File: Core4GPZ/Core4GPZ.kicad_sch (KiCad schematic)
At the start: 3 parts, among them U1 core4, U2 MPX4250

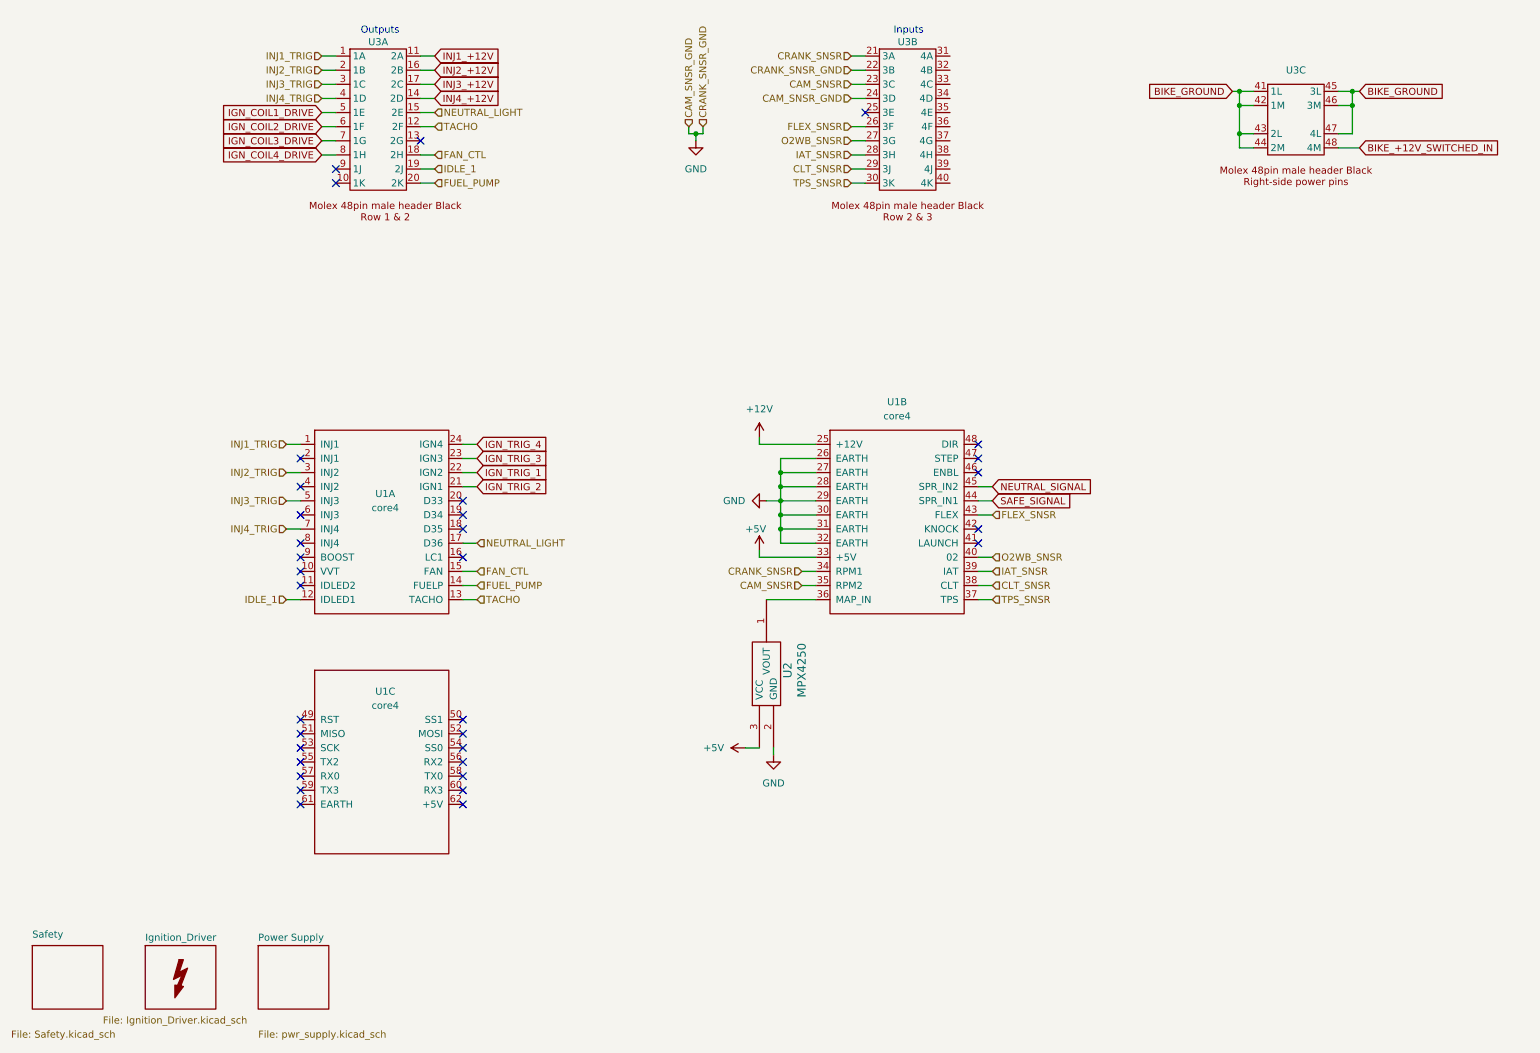
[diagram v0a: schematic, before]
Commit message: Test montage générateur de Haute tension
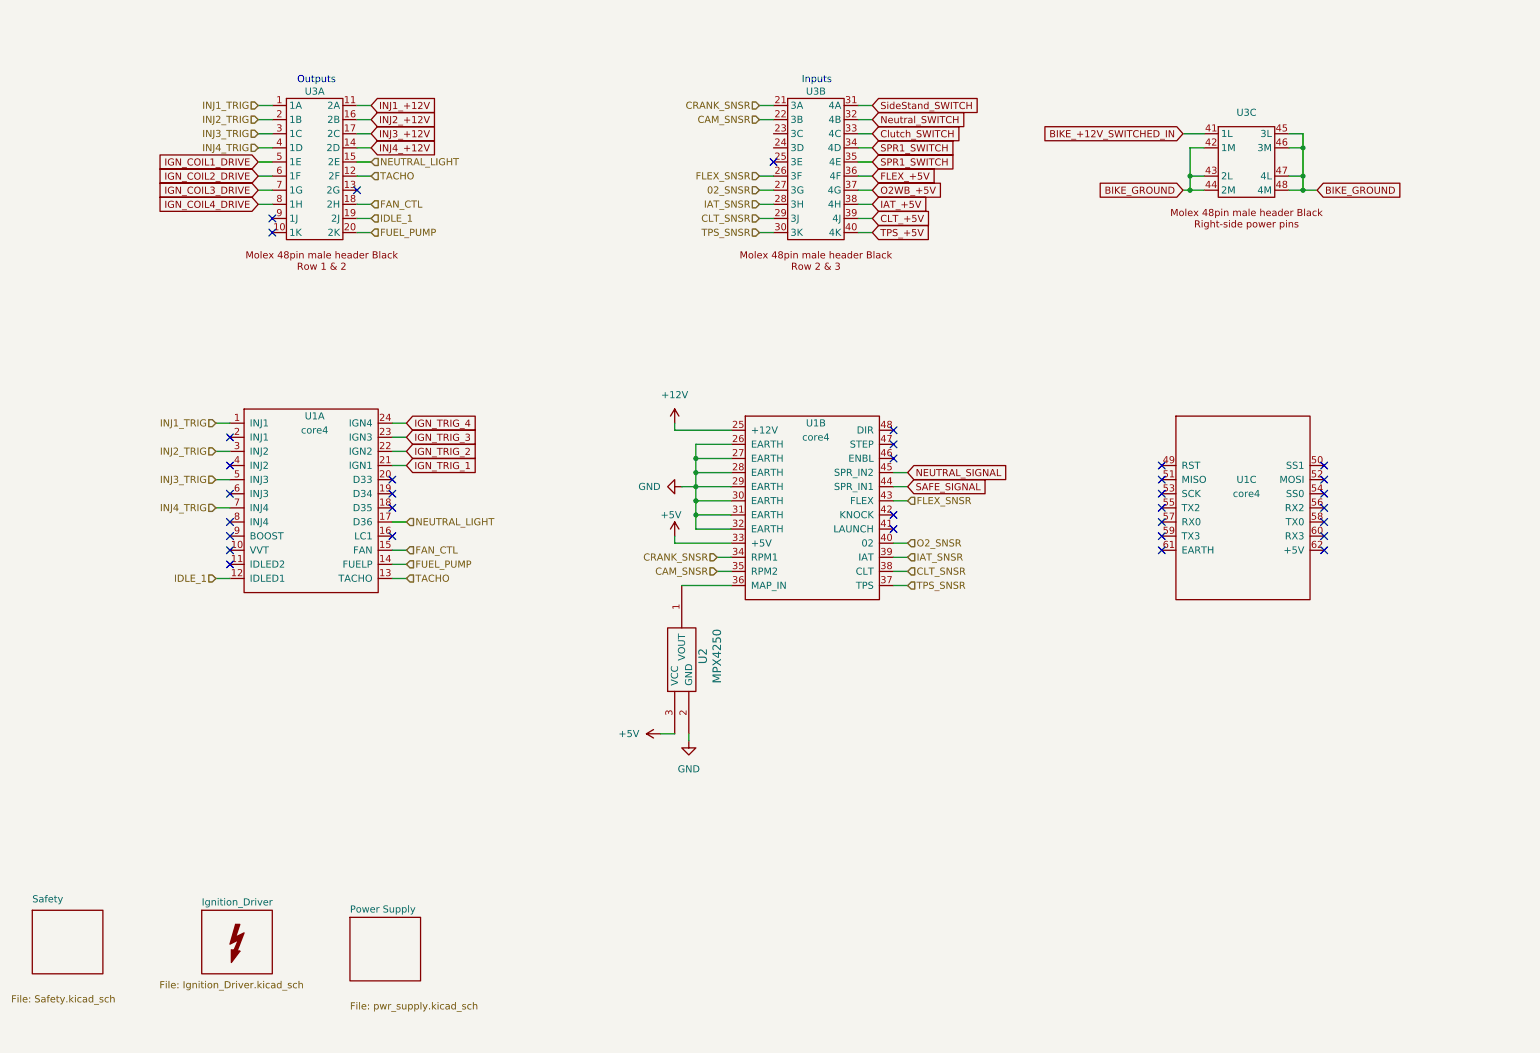
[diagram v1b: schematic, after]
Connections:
- net BIKE_+12V_SWITCHED_IN: now also U3.41 (1L); no longer U3.48 (4M)
- net BIKE_GROUND: now also U3.48 (4M); no longer U3.41 (1L)
- net CAM_SNSR: now also U3.22 (3B); no longer U3.23 (3C)
- net GND: no longer U3.22 (3B), U3.24 (3D)
- net IGN_TRIG_1: now also U1.21 (IGN1); no longer U1.22 (IGN2)
- net IGN_TRIG_2: now also U1.22 (IGN2); no longer U1.21 (IGN1)
- net SideStand_SWITCH: now reaches U3.31 (4A)
- net Neutral_SWITCH: now reaches U3.32 (4B)
- net Clutch_SWITCH: now reaches U3.33 (4C)
- net SPR1_SWITCH: now reaches U3.34 (4D)
- net SPR1_SWITCH: now also U3.35 (4E)
- net FLEX_+5V: now reaches U3.36 (4F)
- net O2WB_+5V: now reaches U3.37 (4G)
- net IAT_+5V: now reaches U3.38 (4H)
- net CLT_+5V: now reaches U3.39 (4J)
- net TPS_+5V: now reaches U3.40 (4K)
- net O2WB_SNSR renamed 02_SNSR
- net 02_SNSR: no longer U1.40 (02)
- new net O2_SNSR: U1.40 (02)
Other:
- moved on the sheet: U1A, U1B, U1C, U2, U3A, U3B, U3C
